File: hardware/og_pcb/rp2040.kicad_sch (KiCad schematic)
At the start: 28 parts, among them J2 Conn_02x03_Top_Bottom, SW4 SW_Push_Shielded, SW5 SW_Push_Shielded, U1 254, U12 RP2040, U3 W25Q128JVS, Y3 ABM8-272-T3

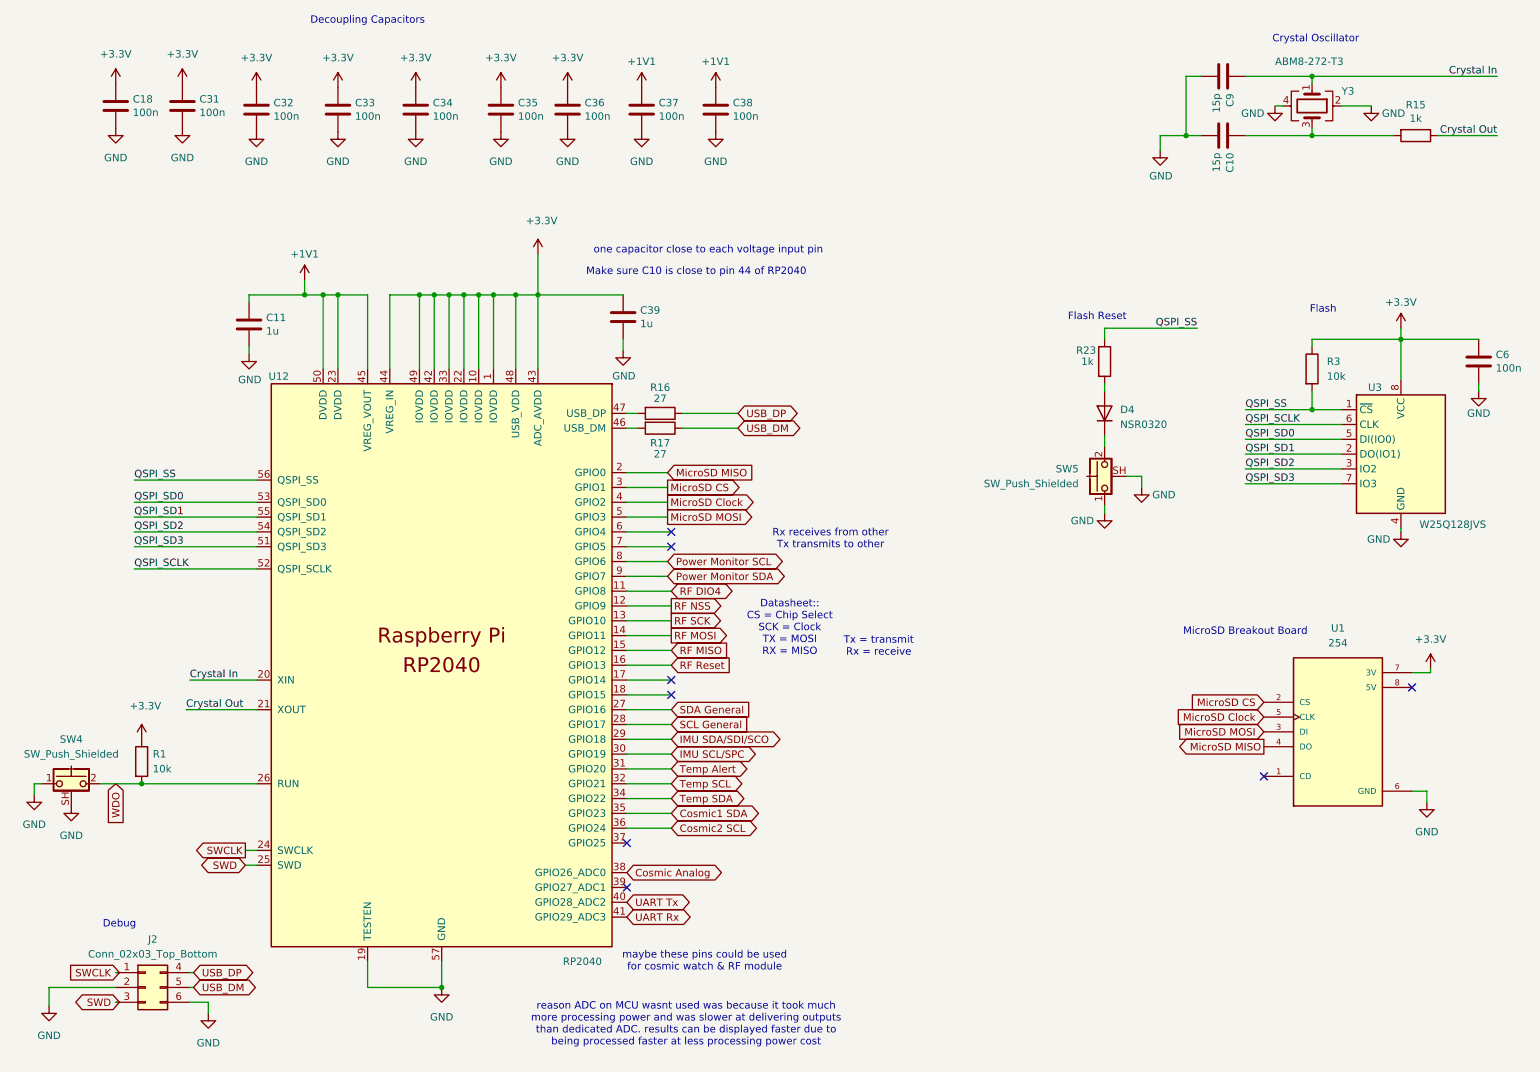
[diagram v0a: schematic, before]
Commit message: updated pcb work in progress (incomplete)
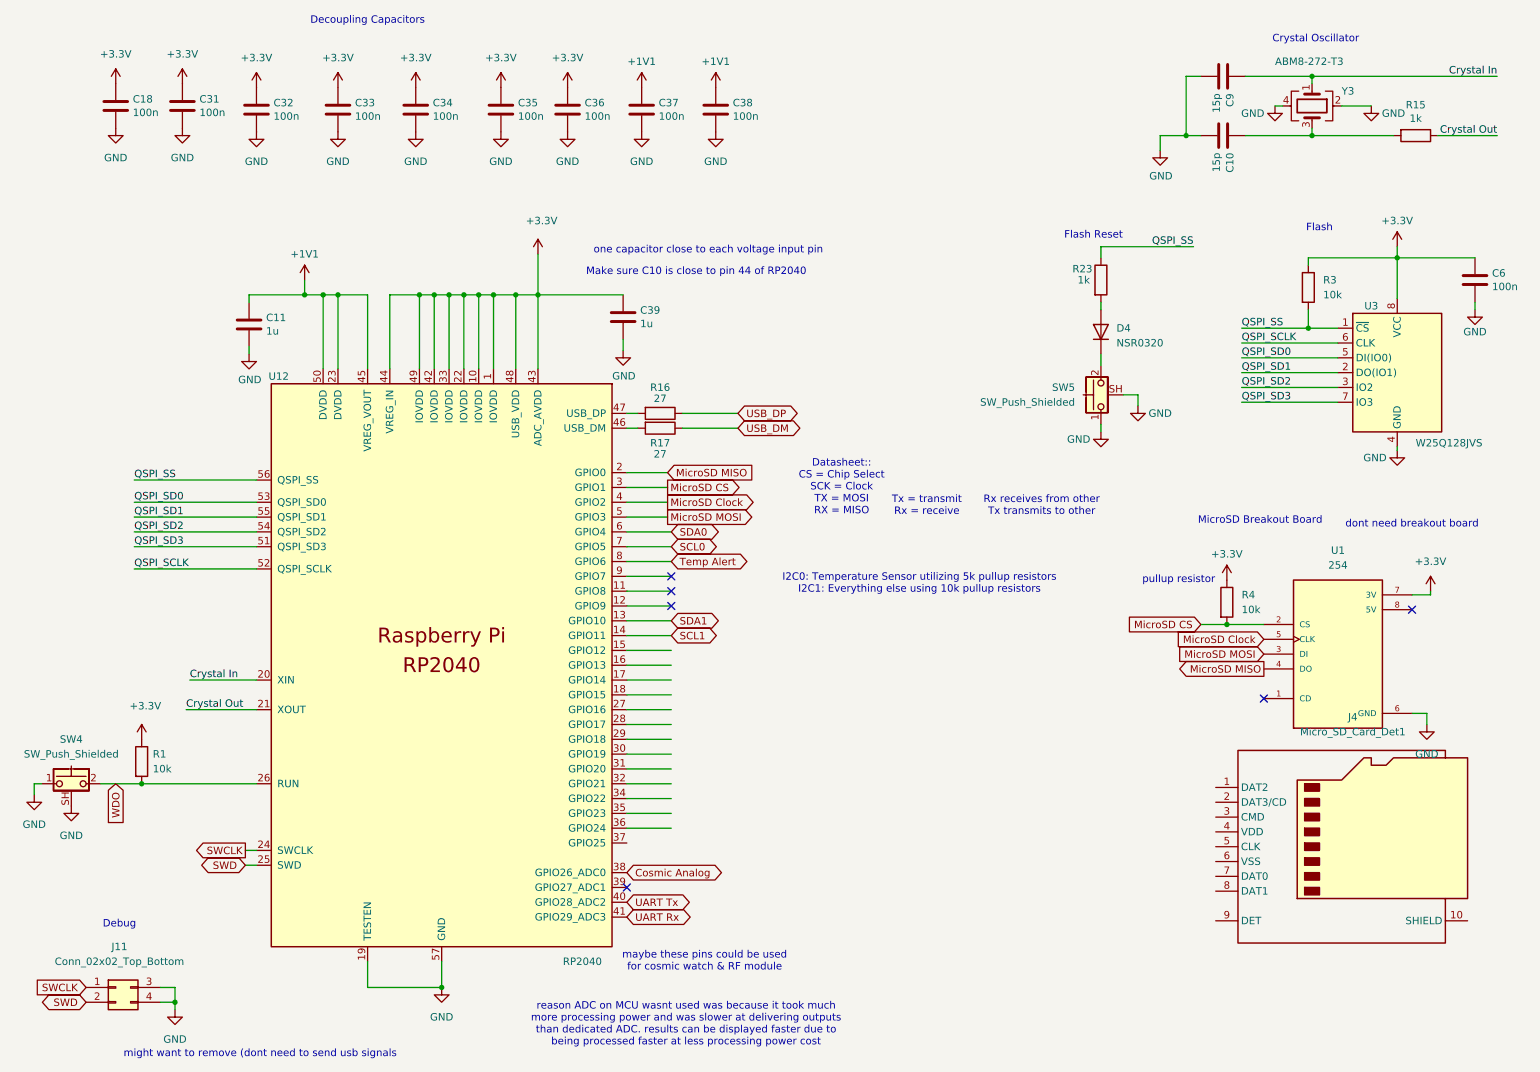
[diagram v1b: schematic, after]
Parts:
- removed J2: Conn_02x03_Top_Bottom, Connector_Hirose:Hirose_DF11-6DP-2DSA_2x03_P2.00mm_Vertical, symbol Connector_Generic:Conn_02x03_Top_Bottom
- added J11: Conn_02x02_Top_Bottom, 1my_footprints:CON4_2X2_UF_DF11_HIR, symbol Connector_Generic:Conn_02x02_Top_Bottom
- added J4: Micro_SD_Card_Det1, symbol Connector:Micro_SD_Card_Det1
- added R4: 10k, Resistor_SMD:R_0402_1005Metric, symbol Device:R
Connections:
- net Power Monitor SCL is gone; now on net Temp Alert: U12.8 (GPIO6)
- net +3.3V: now also R4.1
- net GND: now also J11.3 (Pin_3), J11.4 (Pin_4)
- net MicroSD CS: now also R4.2
- net SWCLK: now also J11.1 (Pin_1)
- net SWD: now also J11.2 (Pin_2)
- net Temp Alert: no longer U12.31 (GPIO20)
- net SDA0: now reaches U12.6 (GPIO4)
- net SCL0: now reaches U12.7 (GPIO5)
- net Cosmic1 SDA: no longer names the net of U12.35 (GPIO23)
- net Cosmic2 SCL: no longer names the net of U12.36 (GPIO24)
- net IMU SCL/SPC: no longer names the net of U12.30 (GPIO19)
- net IMU SDA/SDI/SCO: no longer names the net of U12.29 (GPIO18)
- net Power Monitor SDA: no longer names the net of U12.9 (GPIO7)
- net RF DIO4: no longer names the net of U12.11 (GPIO8)
- net RF MISO: no longer names the net of U12.15 (GPIO12)
- net RF MOSI renamed SCL1
- net RF NSS: no longer names the net of U12.12 (GPIO9)
- net RF Reset: no longer names the net of U12.16 (GPIO13)
- net RF SCK renamed SDA1
- net SCL General: no longer names the net of U12.28 (GPIO17)
- net SDA General: no longer names the net of U12.27 (GPIO16)
- net Temp SCL: no longer names the net of U12.32 (GPIO21)
- net Temp SDA: no longer names the net of U12.34 (GPIO22)
- no-connect marks 8 -> 6
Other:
- note added: "I2C0: Temperature Sensor utilizing 5k pullup resistors I2C1: Everything else using 10k pullup resistors"
- note added: "dont need breakout board"
- note added: "might want to remove (dont need to send usb signals"
- note added: "pullup resistor"
- moved on the sheet: C6, D4, R23, R3, SW5, U1, U3
